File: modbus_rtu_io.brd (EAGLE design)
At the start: 108 x 67.9 mm, 72 parts, among them IC1 MAX3485ESA, IC5 ATMEGA48/88/168-PU, K1 AQY27SMD, K2 AQY22SOP, K3 G6D-1A-ASI12VDC, K4 RP418005, K5 AQG12105, K6 RP418005, K8 AQY22SOP, T1 BC846, T2 BC846, T4 BC846

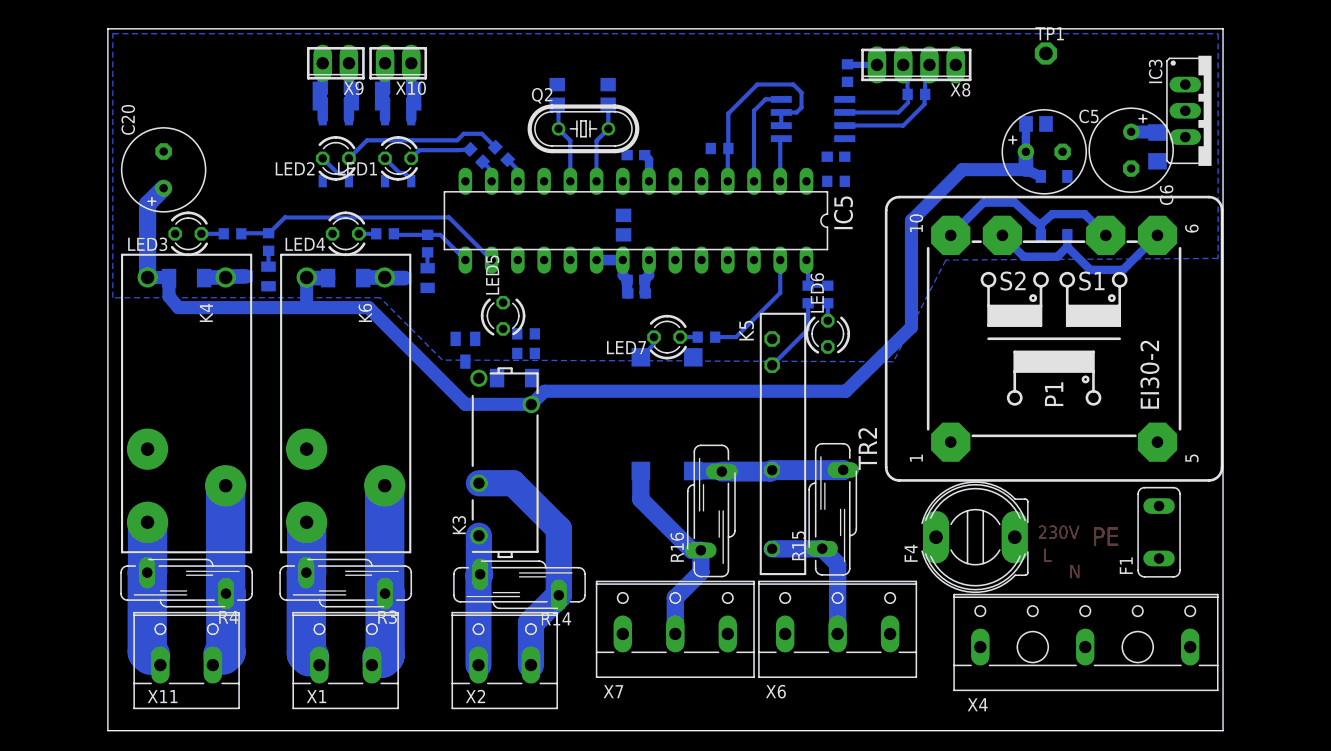
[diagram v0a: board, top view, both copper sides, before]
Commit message: routing fertig
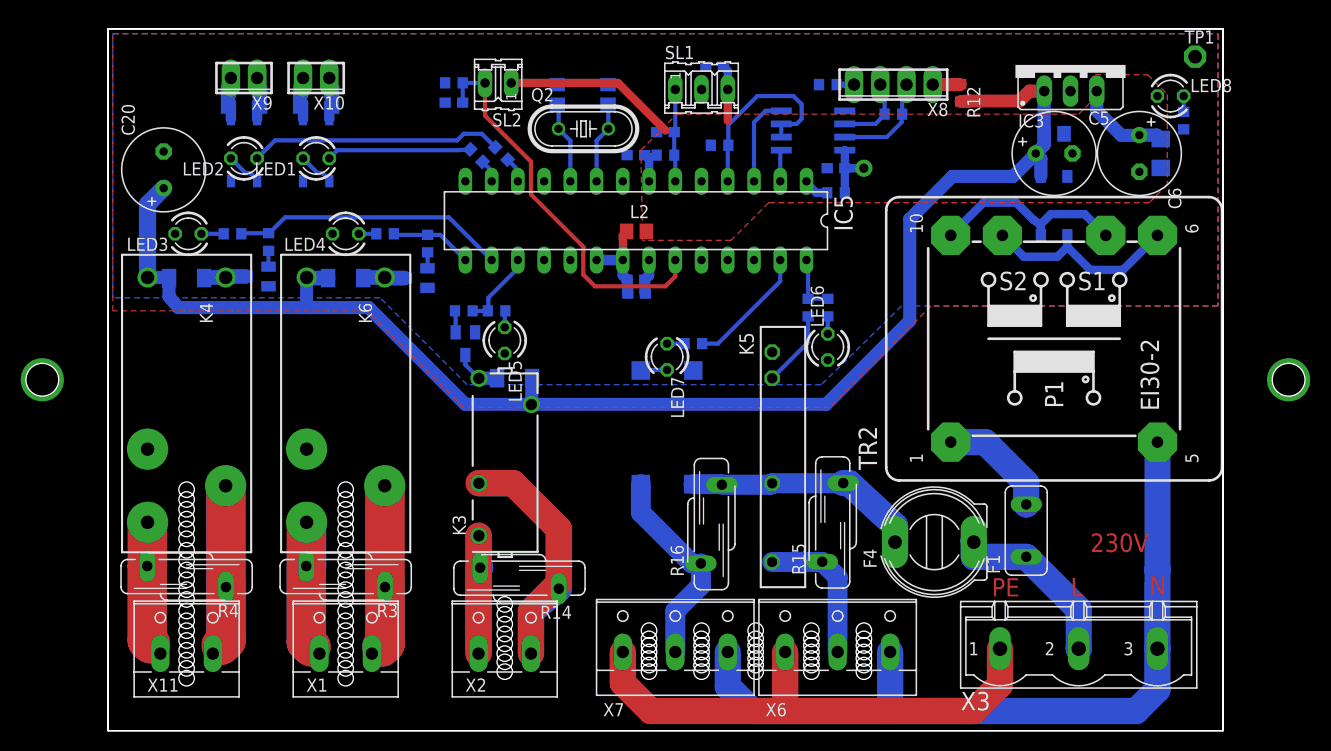
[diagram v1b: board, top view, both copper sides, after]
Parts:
- removed X4: (no value), con-wago-508:W237-3N
- added C3, C7, C8: 100nF, rcl:C0603
- added LED8: (no value), led:LED3MM
- added R12, R23, R24: 120, rcl:R0603
- added R22: 10K, rcl:R0603
- added SL1: (no value), con-amp-quick:03P
- added SL2: (no value), con-amp-quick:02P
- added X3: GMSTBV3, con-phoenix-762:GMSTBV3
- moved TP1 14.4 mm to (105.3, 65.2)
- moved IC3 14.4 mm to (93.2, 64.5), turned to 0 degrees
- moved F1 12.9 mm to (88.9, 19.4)
- moved X9 9.00 mm to (13.2, 63.2)
- moved R17 8.90 mm to (13.2, 61.1)
- moved K2 8.89 mm to (13.2, 56.2)
- moved LED2 8.89 mm to (13.2, 55.4)
- moved X10 8.07 mm to (20.2, 63.2)
- moved R18 7.94 mm to (20.2, 61.1)
- moved K8 7.94 mm to (20.2, 56.2)
- moved LED1 7.94 mm to (20.2, 55.4)
- moved R9 7.31 mm to (34.4, 40.6)
- moved F4 4.00 mm to (80.0, 18.3)
- moved R30 3.62 mm to (37.6, 40.6), turned to 180 degrees
- moved R1 2.93 mm to (76.0, 59.7)
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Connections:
- new net N$45: R12.1, X8.1
- new net N$51: LED8.K, R22.2
- new net N$53: C7.1, IC5.6, R23.1, SL1.1
- new net N$56: C8.2, IC5.23, R24.2, SL2.2
- net +12V: now also R12.2
- net +5V: now also C3.1, LED8.A, R23.2, SL1.3, SL2.1
- net GND: now also C3.2, C7.2, C8.1, R22.1, R24.1, SL1.2
- net L: now also X3.2; no longer X4.1
- net N$23: now also TR2.1; no longer TR2.5
- net N$28: now also TR2.5, X3.3; no longer TR2.1, X4.2
- net PE: now also X3.1; no longer X4.3
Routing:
- net N$28: track 0.00 -> 76.6 mm
- net PE: track 0.00 -> 51.0 mm
- net N$56: track 0.00 -> 37.9 mm
- net +5V: track 5.26 -> 41.3 mm, vias 0 -> 1
- net N$26: track 23.9 -> 45.7 mm
- net L: track 0.00 -> 18.1 mm
- net N$49: track 0.00 -> 15.7 mm
- net N$47: track 0.00 -> 15.6 mm
- net +12V: track 127.2 -> 142.4 mm
- net N$48: track 0.00 -> 12.3 mm
- net N$46: track 0.00 -> 11.9 mm
- net N$23: track 0.00 -> 11.0 mm
- net N$25: track 12.6 -> 23.0 mm
- net N$53: track 0.00 -> 8.97 mm
- net N$42: track 15.7 -> 24.6 mm
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- added copper zone on layer 1, net +5V
- added copper zone on layer 1, net GND
